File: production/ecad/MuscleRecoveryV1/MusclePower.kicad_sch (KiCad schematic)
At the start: 27 parts, among them IC1 LC709203FQH-01TWG, Q1 FDN340P, U1 AP1117-33, U2 MCP73831-2-OT, U6 ESP32-WROOM-32

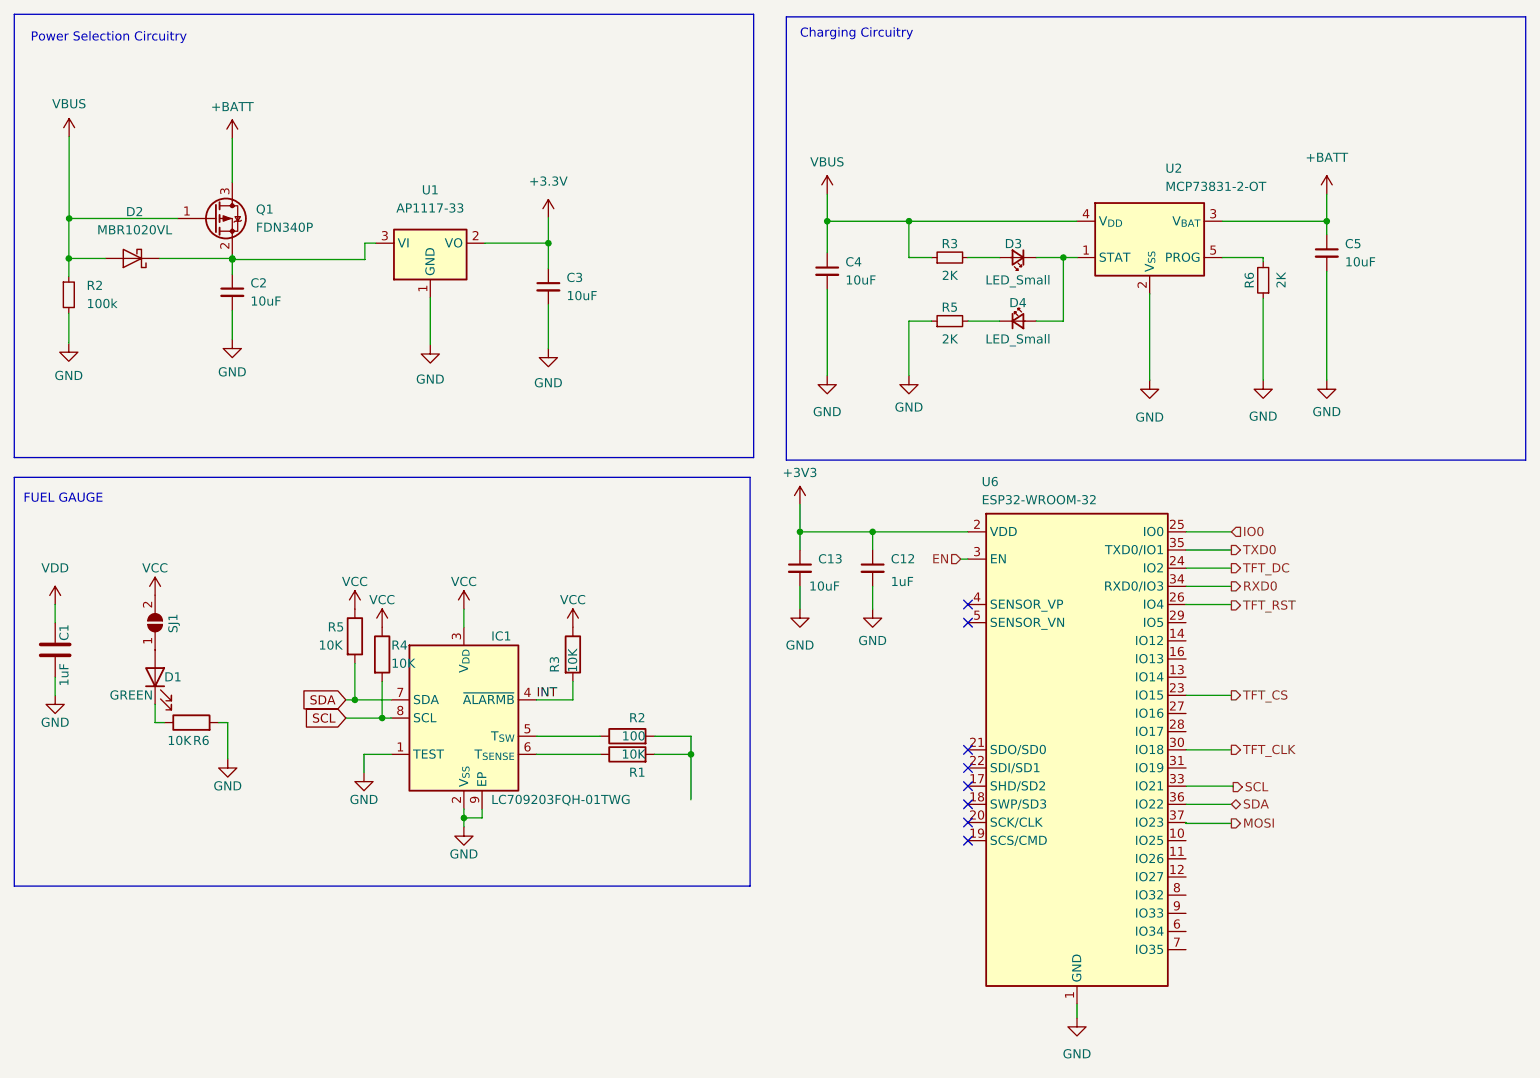
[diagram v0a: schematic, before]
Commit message: Revert "Display commit 1"
This reverts commit 52e50f7827ccbfa861bea7a8a003d131d02fed89.
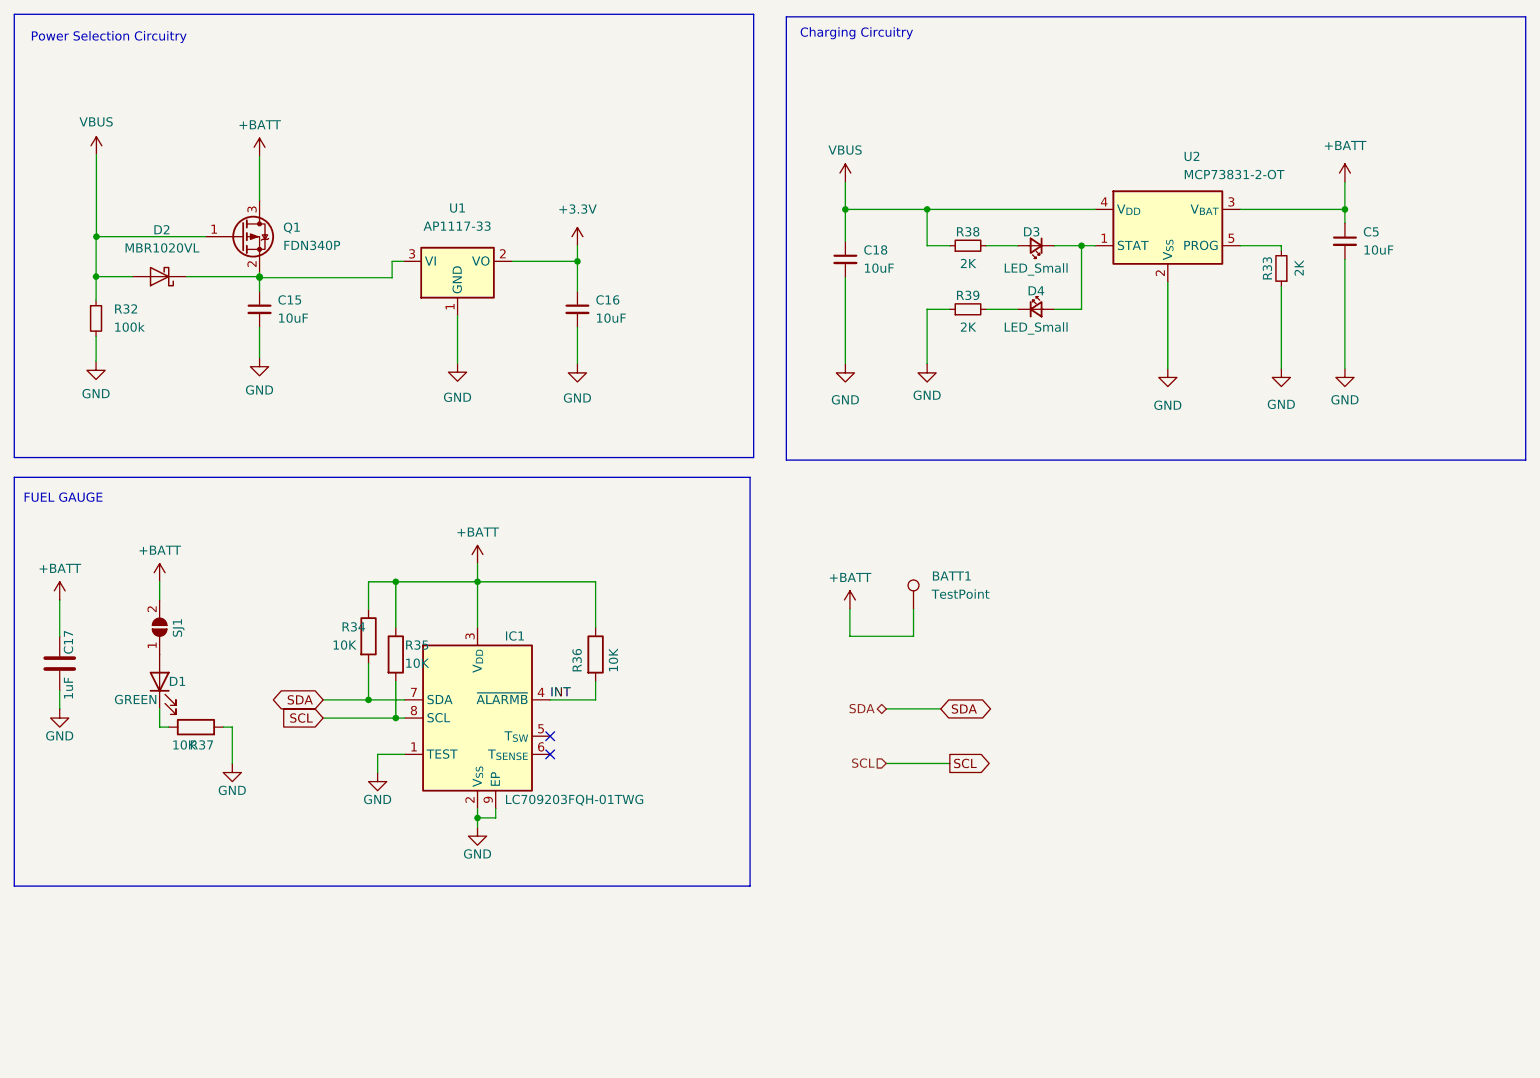
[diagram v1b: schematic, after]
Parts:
- removed C1: 1uF, symbol Device:C
- removed C12: 1uF, symbol Device:C_Small
- removed C13, C2, C3, C4: 10uF, symbol Device:C_Small
- removed R1, R3: 10K, Resistor_SMD:R_0805_2012Metric, symbol Device:R
- removed R2: 100, Resistor_SMD:R_0805_2012Metric, symbol Device:R
- removed R2: 100k, symbol Device:R_Small
- removed R3, R5, R6: 2K, symbol Device:R_Small
- removed R4, R5, R6: 10K, symbol Device:R
- removed U6: ESP32-WROOM-32, RF_Module:ESP32-WROOM-32, symbol RF_Module:ESP32-WROOM-32
- added BATT1: TestPoint, symbol Connector:TestPoint
- added C15, C16, C18: 10uF, symbol Device:C_Small
- added C17: 1uF, symbol Device:C
- added R32: 100k, symbol Device:R_Small
- added R33, R38, R39: 2K, symbol Device:R_Small
- added R34, R35, R37: 10K, symbol Device:R
- added R36: 10K, Resistor_SMD:R_0805_2012Metric, symbol Device:R
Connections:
- net VCC is gone; now on net +BATT: IC1.3 (V_{DD}), SJ1.2 (B)
- net +3.3V: now also C16.1
- net +BATT: now also BATT1.1, C17.1, R34.1, R35.1, R36.1
- net GND: now also C15.2, C16.2, C17.2, C18.2, R32.2, R33.1, R37.2, R39.1
- net INT: now also R36.2
- net SCL: now also R35.2
- net SDA: now also R34.2
- net VBUS: now also C18.1, R32.1, R38.1
- net at D2.1 (K), Q1.2 (S), U1.3 (VI): now also C15.1
- net at D1.1 (K): now also R37.1
- net at D4.1 (K): now also R39.2
- net at D3.2 (A): now also R38.2
- net at U2.5 (PROG): now also R33.2
- no-connect marks 8 -> 2
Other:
- moved on the sheet: D1, D2, D3, D4, IC1, Q1, SJ1, U1, U2
